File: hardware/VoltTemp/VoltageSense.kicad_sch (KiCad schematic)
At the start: 31 parts, among them IC1 ISO1641BDR, SW1 BOOT, U1 EL3H7, U2 BQ7692003PW, U3 EL3H7

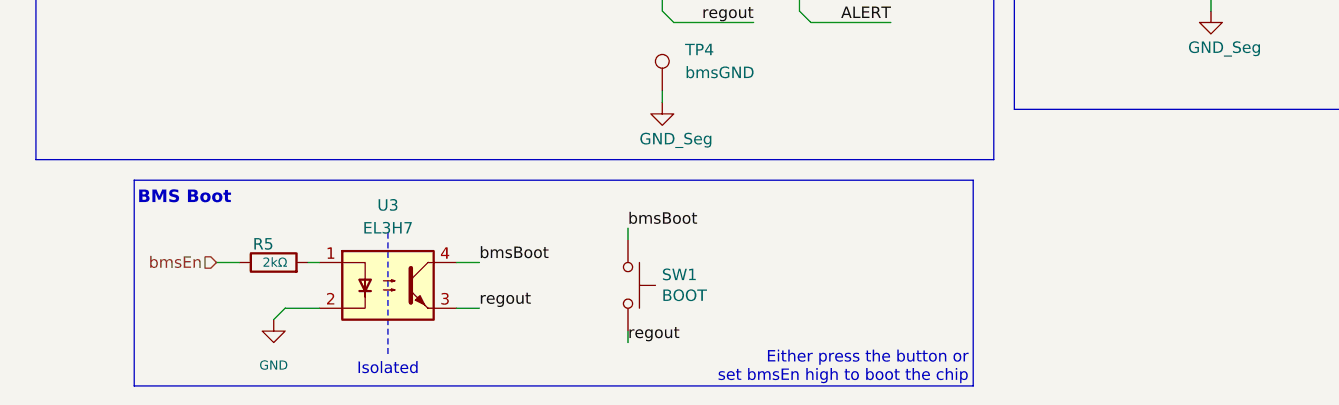
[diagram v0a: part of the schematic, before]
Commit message: Staircase (#6)
* this is the staircase board :(

* I added the 3d models for the connectors. Need to swap layers around some

* Traces finished, passes DRC, need to complete silkscreen

* changes

* Initial board done. Labels on everything, yay

* Goofy pictures and names added

* goofy things

* Review Council concerns have been dealt with :-)

* Boot switch changed to V_Boot, ShieldGND added to scrut conn, labels added to LEDs, misc routing tweaks

* i tweaked one more thing :)

* lakshay concerns dealt with and also i did the jlcpcb generation thing

* fix

* i fixed the clearance violation :-)

* STEP file generated

* board center origin

* ninjafix thanks lakshay :(

* gerbers

* bom

* bom

---------

Co-authored-by: Clark Rucker <clarkrucker@utexas.edu>
Co-authored-by: sodaplayzz <sc.seaofthieves@gmail.com>
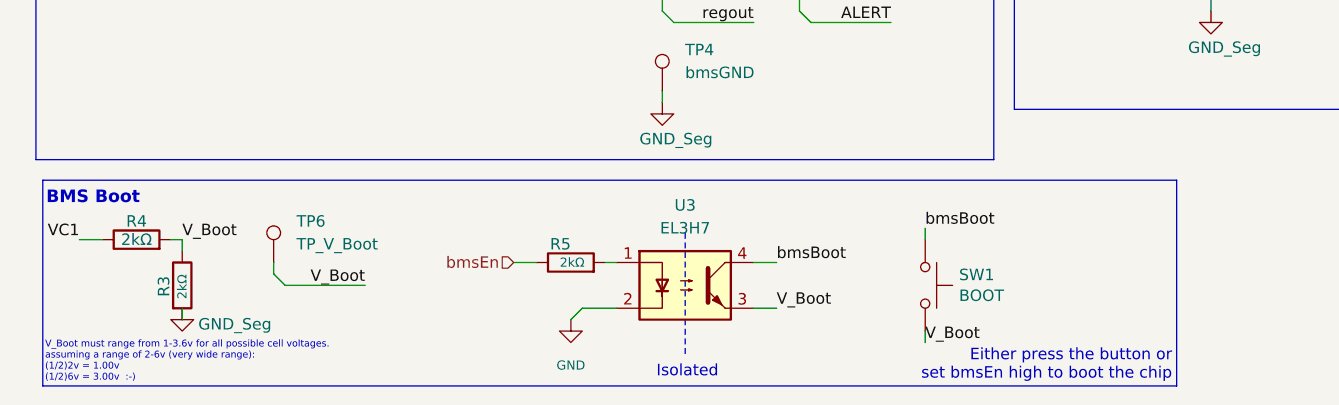
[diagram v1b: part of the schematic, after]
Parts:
- added R3, R4: 2kΩ, Resistor_SMD:R_0603_1608Metric_Pad0.98x0.95mm_HandSolder, symbol Device:R
- added TP6: TP_V_Boot, TestPoint:TestPoint_Pad_1.0x1.0mm, symbol Connector:TestPoint
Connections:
- net GND_Seg: now also R3.2
- net VC1: now also R4.1
- net regout: no longer SW1.2, U3.3
- new net V_Boot: R3.1, R4.2, SW1.2, TP6.1, U3.3
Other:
- note added: "V_Boot must range from 1-3.6v for all possible cell voltages. assuming a range of 2-6v (very wide range): (1/2)2v = 1.00v (1/2)6v = 3.00v :-)"
- moved on the sheet: R5, SW1, U3
